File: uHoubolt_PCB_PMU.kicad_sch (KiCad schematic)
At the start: 118 parts, among them J10 Debug, J11 AltimaxPwr, J12 CAN1, J13 CAN2, J14 CAN1, J15 CAN2, J16 CAN1, J17 CAN2, J18 CAN1, J19 CAN2, J2 Battery, J23 Payload, J25 RCU, J27 Umbilical0, J28 Umbilical0, J29 AltimaxArm, J3 Power, J4 BatteryAltimax, J5 Umbilical1, J6 AltimaxArm, J8 Altimax_PWR, J9 Debug, Q1 BSZ0905PNSATMA1, Q2 BSZ0902NSATMA1, Q3 SISA88DN or similar, SW1 Power_1, SW2 Power_2, SW3 Pyro_1, SW4 Pyro_2, U1 LM5069, U10 ICM-20602, U11 LPS25HB, U12 SFH617A-1X007T, U14 LiIon_Charger, U15 SFH617A-1X007T, U2 LMP8640 F, U4 LiIon_Charger, U5 STM32G491MET6-LQFP80, U6 W25Q256JV, U7 MCP1700-3302E, U8 MCP2562FDx-x_MF, U9 MCP2562FDx-x_MF, X1 TXC-7C

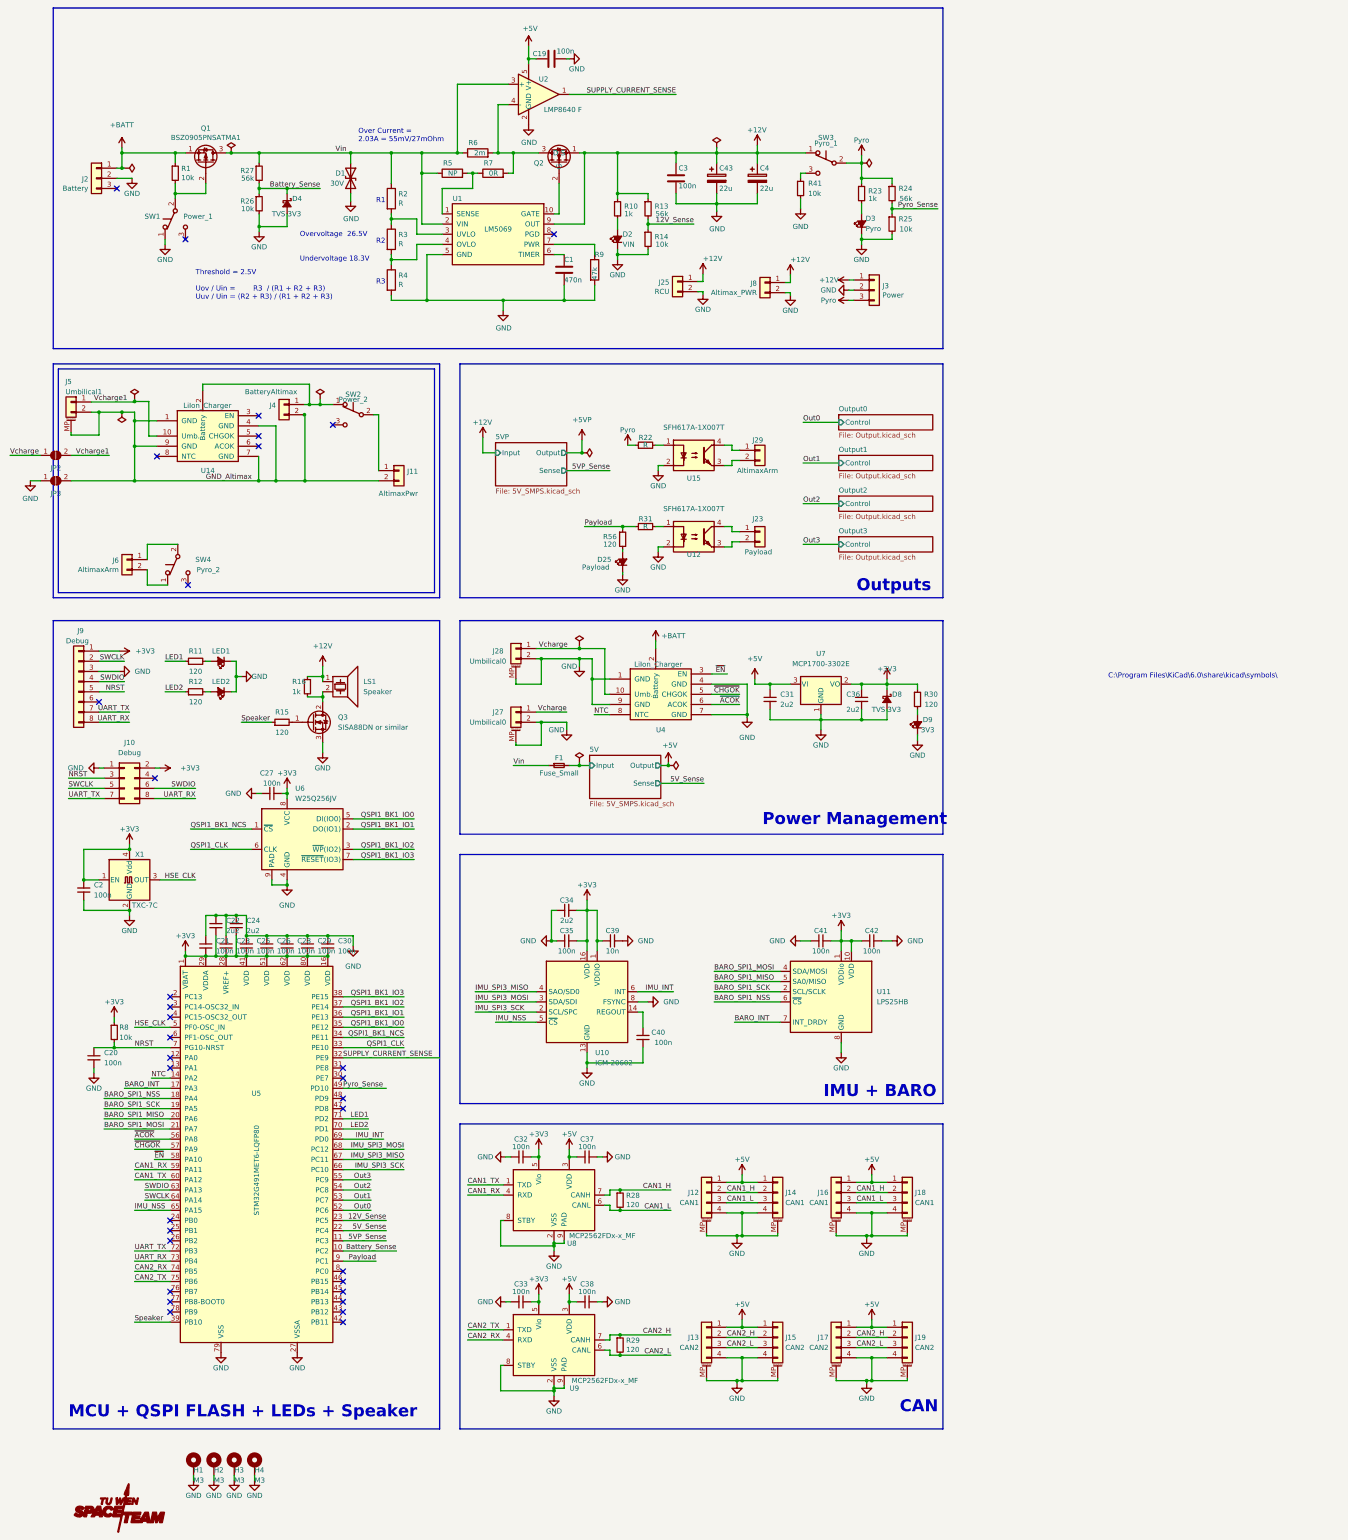
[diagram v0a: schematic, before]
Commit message: Revert "PMU V3 "ready to order?""
This reverts commit e5aaef69110c3557dfda333950fee24891806424.
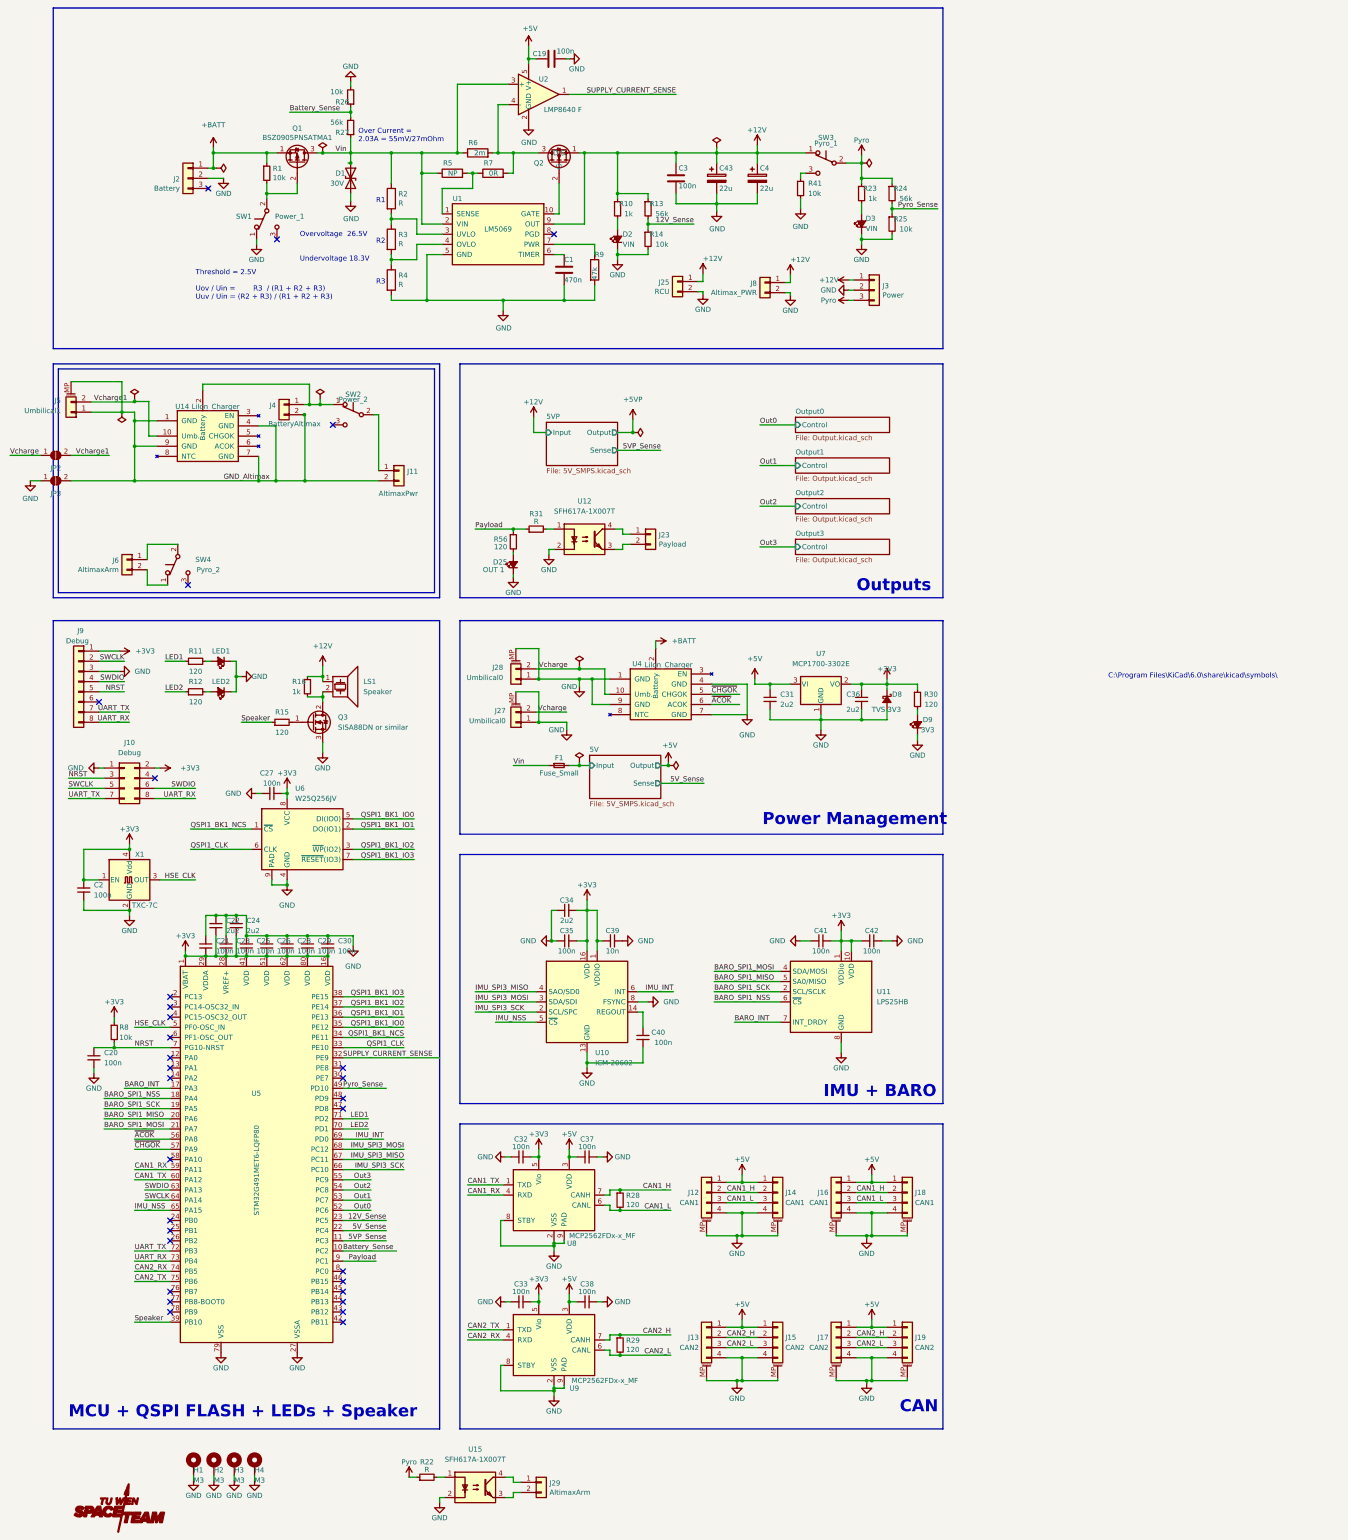
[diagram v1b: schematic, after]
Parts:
- removed D4: TVS 3V3, TXV_Library_Footprints:SOD882D, symbol Device:D_Schottky_Small_Filled
- D25: value Payload -> OUT 1
- D3: value Pyro -> VIN
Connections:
- net Vcharge is gone; now on net GND: J27.1 (Pin_1), J28.1 (Pin_1), JP2.1 (A), U4.10 (Umb.)
- net GND_Altimax: now also J5.1 (Pin_1); no longer J5.2 (Pin_2)
- net Vcharge1: now also J5.2 (Pin_2); no longer J5.1 (Pin_1)
- net NTC: no longer names the net of U5.14 (PA2)
- net NTC: no longer U4.8 (NTC)
- net ~{EN}: no longer names the net of U5.58 (PA10)
- net ~{EN}: no longer U4.3 (EN)
- no-connect marks 33 -> 31
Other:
- moved on the sheet: D25, J2, J23, J27, J28, J29, J5, Q1, R1, R22, R26, R27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

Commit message: PMU V3 "ready to order?"
ready to validate changes
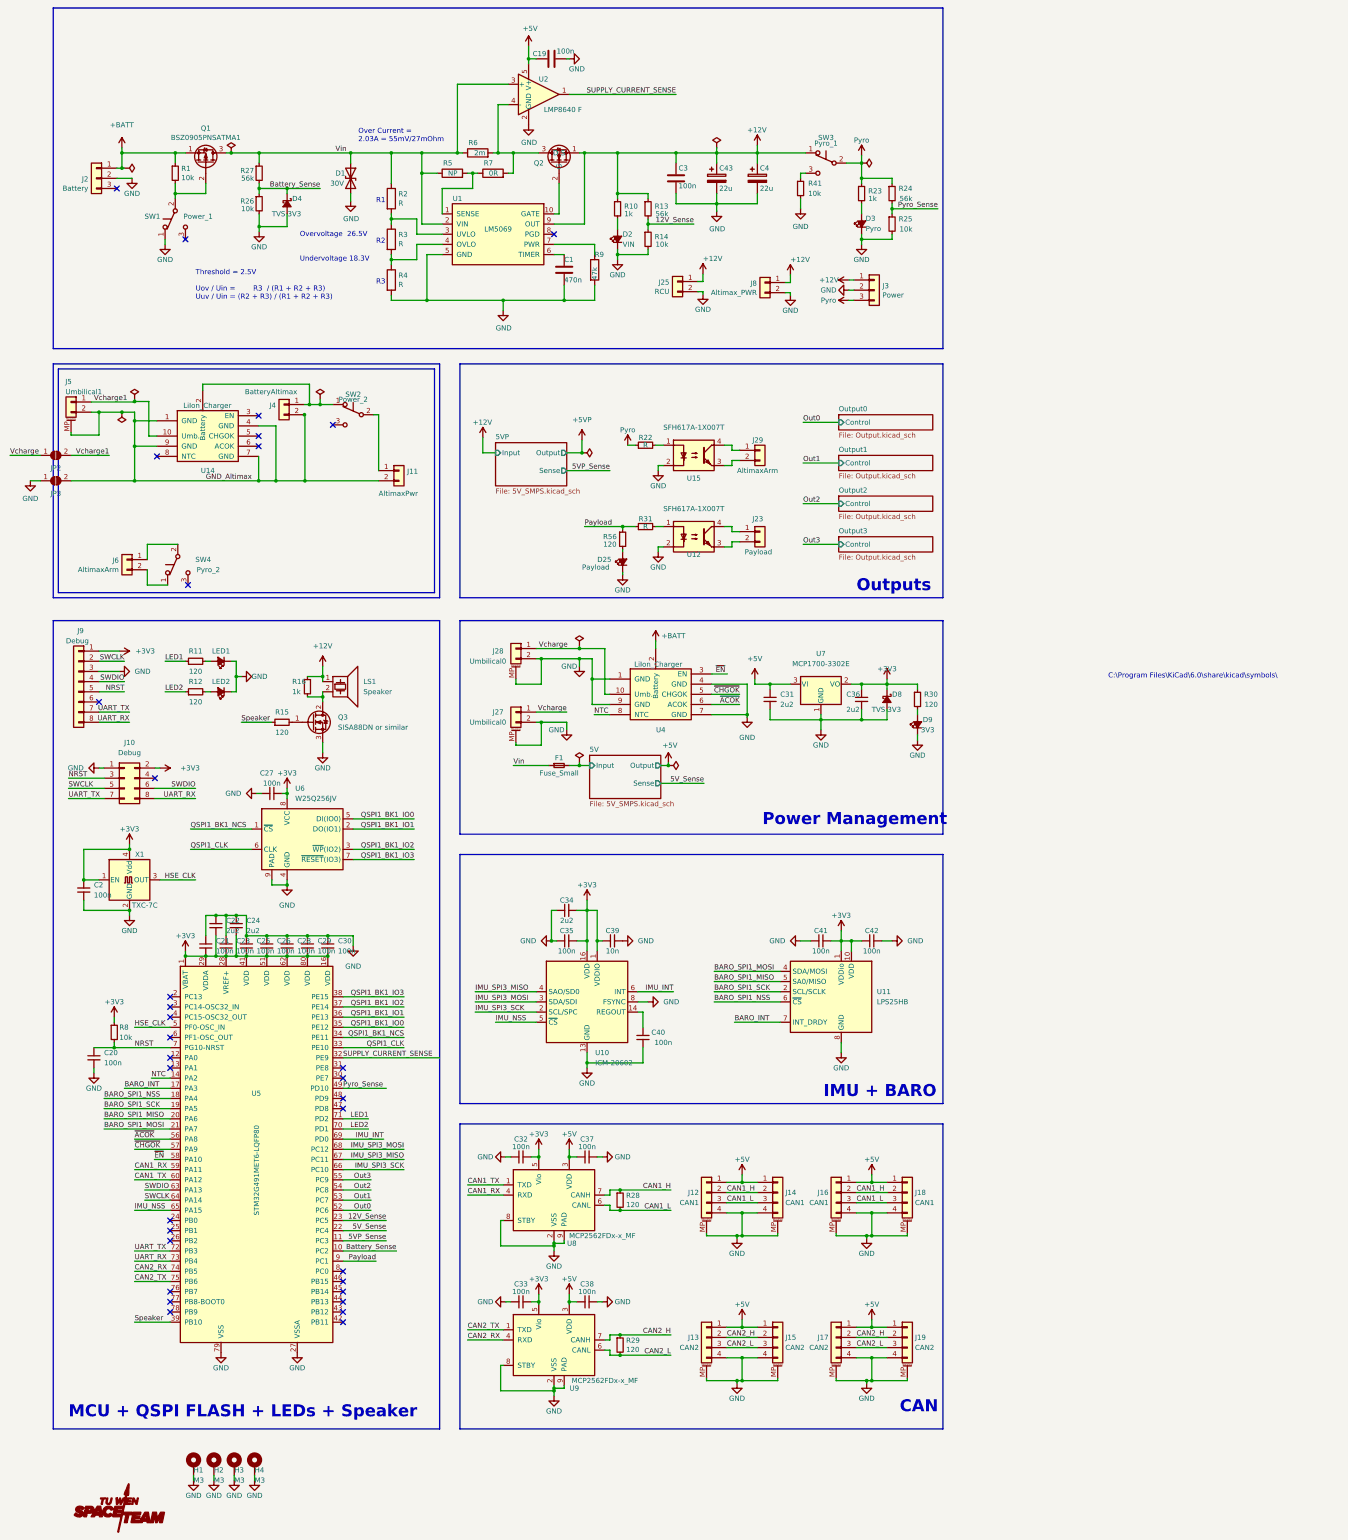
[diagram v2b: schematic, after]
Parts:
- added D4: TVS 3V3, TXV_Library_Footprints:SOD882D, symbol Device:D_Schottky_Small_Filled
- D25: value OUT 1 -> Payload
- D3: value VIN -> Pyro
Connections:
- net Battery_Sense: now also D4.1 (K)
- net GND: now also D4.2 (A); no longer J27.1 (Pin_1), J28.1 (Pin_1), JP2.1 (A), U4.10 (Umb.)
- net GND_Altimax: now also J5.2 (Pin_2); no longer J5.1 (Pin_1)
- net Vcharge1: now also J5.1 (Pin_1); no longer J5.2 (Pin_2)
- net NTC: now reaches U5.14 (PA2)
- net NTC: now also U4.8 (NTC)
- net ~{EN}: now reaches U5.58 (PA10)
- net ~{EN}: now also U4.3 (EN)
- new net Vcharge: J27.1 (Pin_1), J28.1 (Pin_1), JP2.1 (A), U4.10 (Umb.)
- no-connect marks 31 -> 33
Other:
- moved on the sheet: D25, J2, J23, J27, J28, J29, J5, Q1, R1, R22, R26, R27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
